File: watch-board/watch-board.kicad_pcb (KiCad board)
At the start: 2 copper layers, 34 x 34 mm, 64 parts, among them J1 Conn_PAD, J2 Conn_PAD, J3 Conn_PAD, J4 Conn_PAD, J5 Conn_PAD, Q1 Phototransistor_ALS-PT19-315C, Q2 Phototransistor_ALS-PT19-315C, Q3 Transistor_MMBT3904-TP, U1 Display-Driver_PCA8561ANH, U2 Regulator_BQ25504, U3 Regulator_LTC3531-3, U4 MCU_STM32L051K8Ux

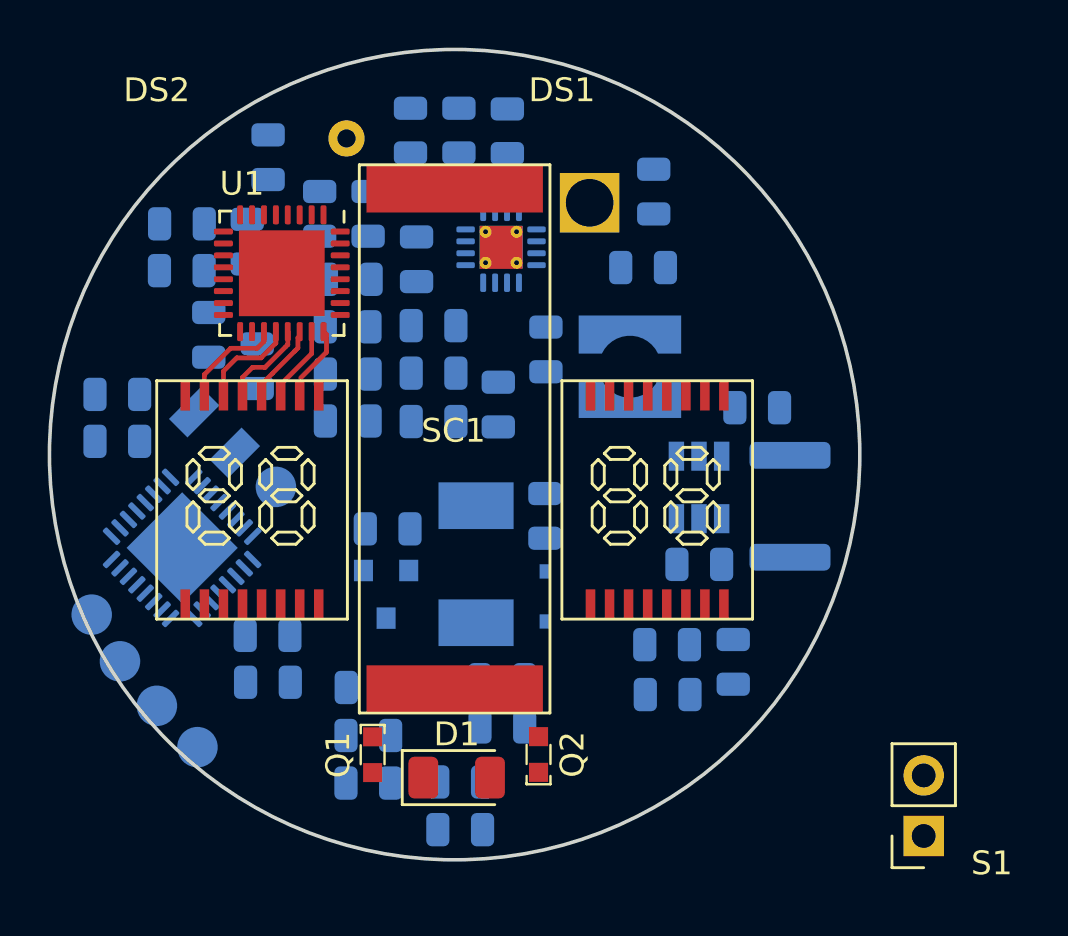
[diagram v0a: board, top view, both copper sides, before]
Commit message: LCDs fully wired :)
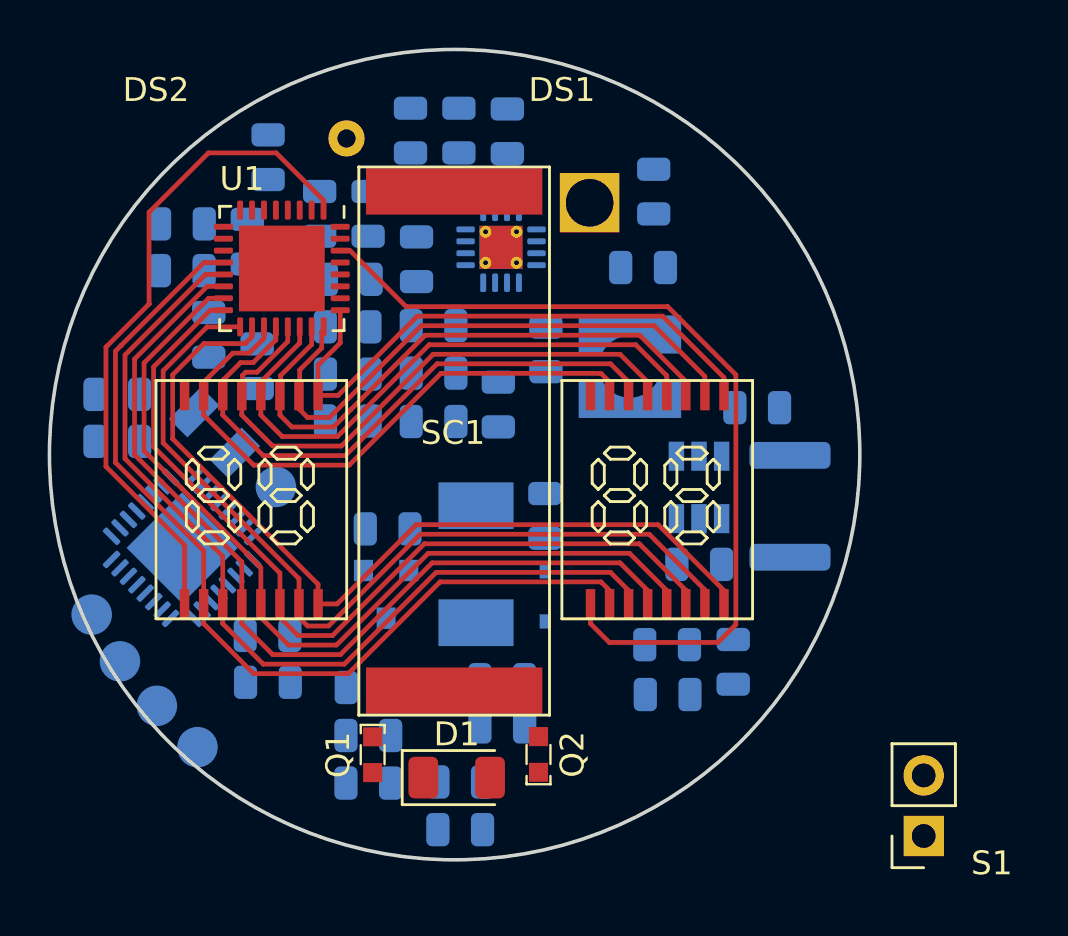
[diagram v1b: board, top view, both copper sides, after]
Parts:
- moved U1 0.20 mm to (132.8, 92.2)
- moved SC1 0.09 mm to (140.0, 99.4)
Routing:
- net /1G: track 0.00 -> 39.2 mm
- net /1F: track 0.00 -> 38.7 mm
- net /1E: track 0.00 -> 38.2 mm
- net /1D: track 0.00 -> 37.5 mm
- net /1B: track 0.00 -> 37.0 mm
- net /1C: track 0.00 -> 36.9 mm
- net /COM1: track 0.00 -> 36.8 mm
- net /1A: track 0.00 -> 36.7 mm
- net /COM2: track 0.00 -> 28.1 mm
- net /2G: track 0.00 -> 24.2 mm
- net /2F: track 2.45 -> 24.3 mm
- net /2E: track 2.76 -> 24.4 mm
- net /2D: track 3.31 -> 24.7 mm
- net /2C: track 3.58 -> 25.0 mm
- net /2B: track 3.99 -> 25.1 mm
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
